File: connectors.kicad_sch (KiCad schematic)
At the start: 30 parts, among them J10 Conn_01x06, J11 Conn_01x04, J12 USB_C_Receptacle_USB2.0_16P, J14 Conn_01x03, J6 FTSH-107-01-L-DV-K-TR, J7 Conn_01x03, J8 Conn_01x02, J9 Conn_01x07, Q7 Si2302CDS

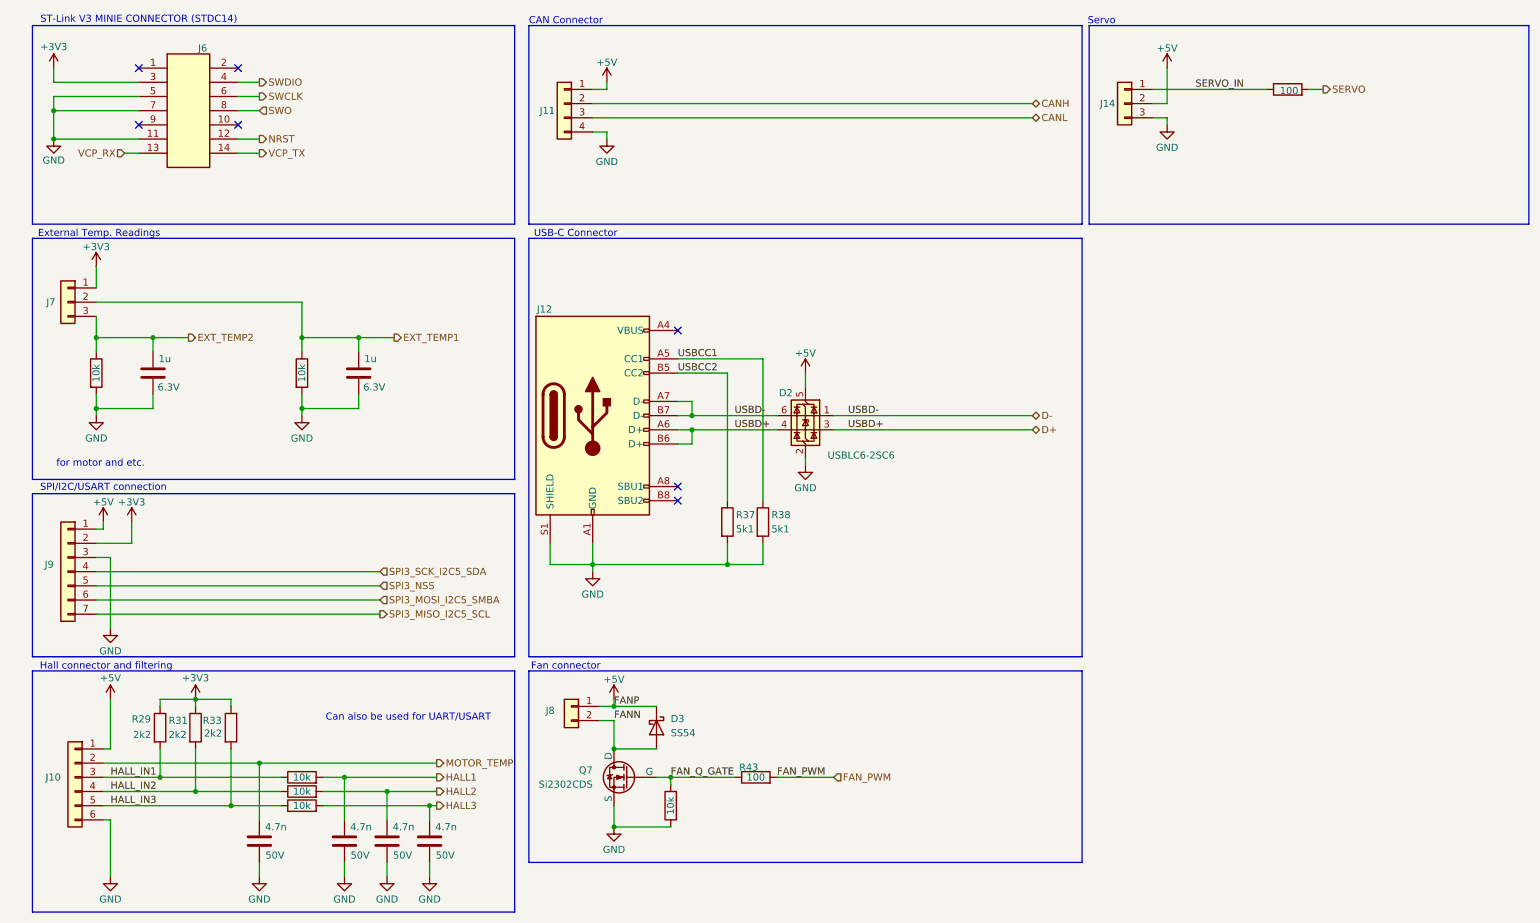
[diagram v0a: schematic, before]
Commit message: wip second draft of the PCB
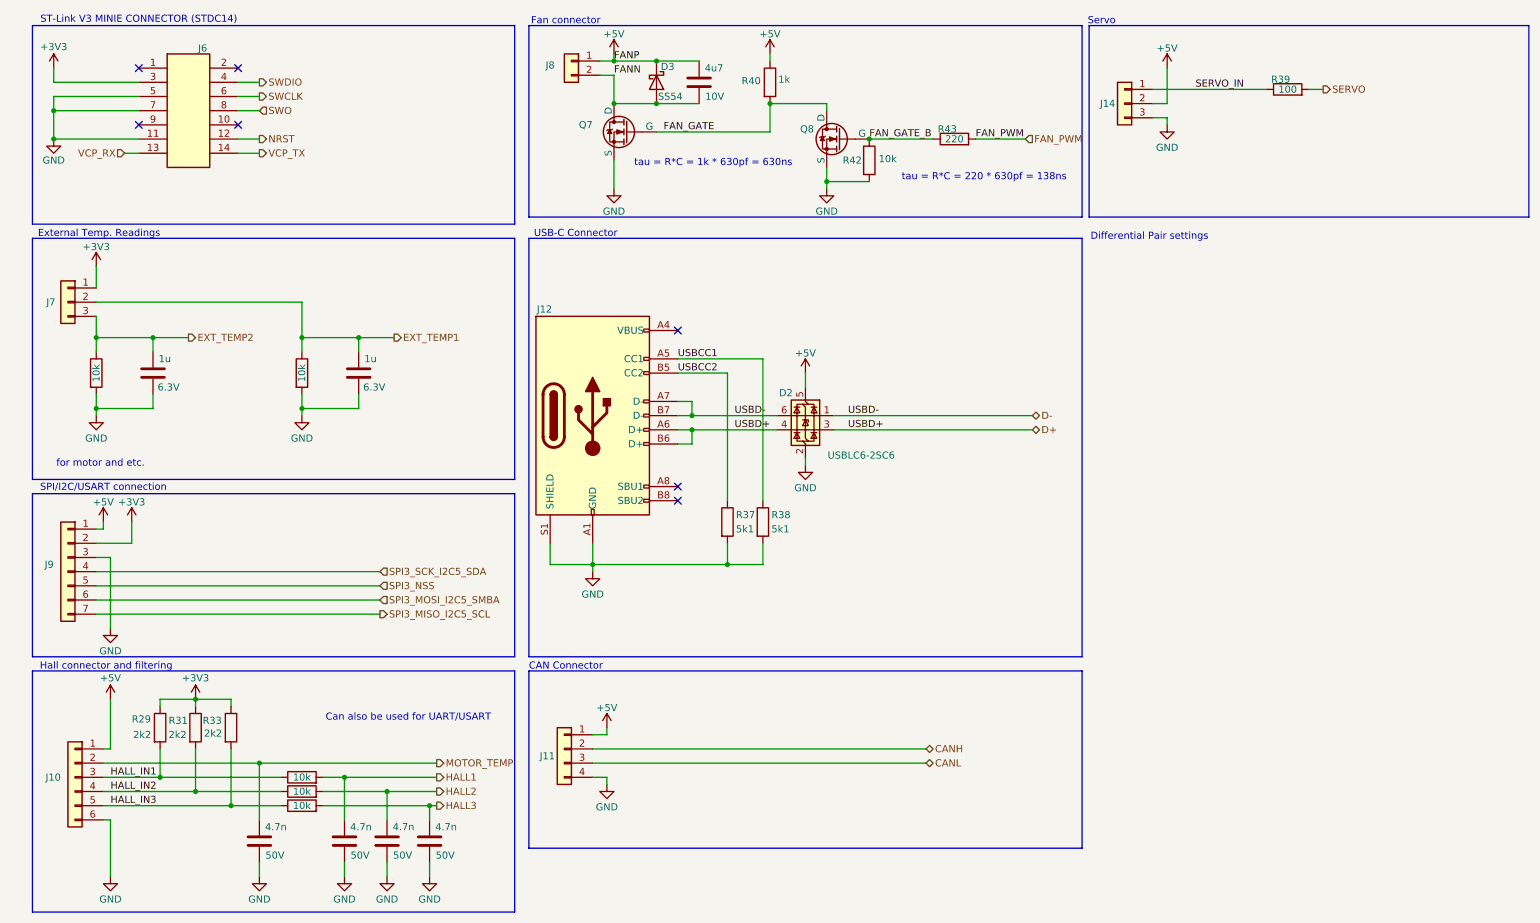
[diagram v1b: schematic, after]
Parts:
- removed R50: 100, Resistor_SMD:R_0402_1005Metric, symbol Device:R
- added C93: 4u7, Capacitor_SMD:C_0402_1005Metric, symbol Device:C
- added Q8: AO3400A, NanoGaN:SOT-23_3, symbol Simulation_SPICE:NMOS
- added R39: 0402WGF1000TCE, Resistor_SMD:R_0402_1005Metric, symbol Device:R
- added R40: 0402WGF1001TCE, Resistor_SMD:R_0402_1005Metric, symbol NanoGaN:R
- Q7: value Si2302CDS -> AO3400A; footprint NanoGaN:SOT-23_Si2302CDS -> NanoGaN:SOT-23_3; LCSC C10488 -> (none)
- R42: value 10k -> 0402WGF1002TCE; Resistance (none) -> 10k
- R43: value 100 -> 0402WGF2200TCE; LCSC C25076 -> C25091; Resistance (none) -> 220
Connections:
- net +5V: now also C93.1, R40.1
- net FANN: now also C93.2
- net GND: now also R42.2, Q8.3 (S); no longer R42.1
- net SERVO: now also R39.2
- net SERVO_IN: now also R39.1
- removed net FAN_Q_GATE: Q7.2 (G), R42.2, R43.1
- new net FAN_GATE: Q7.2 (G), Q8.1 (D), R40.2
- new net FAN_GATE_B: Q8.2 (G), R42.1, R43.1
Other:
- note added: "Differential Pair settings"
- note added: "tau = R*C = 1k * 630pf = 630ns"
- note added: "tau = R*C = 220 * 630pf = 138ns"
- moved on the sheet: D3, J11, J8, R43
